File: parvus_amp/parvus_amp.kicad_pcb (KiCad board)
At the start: 2 copper layers, 86 x 60 mm, 43 parts, among them J1 input, J2 output, J3 powersupply, U1 LM3886

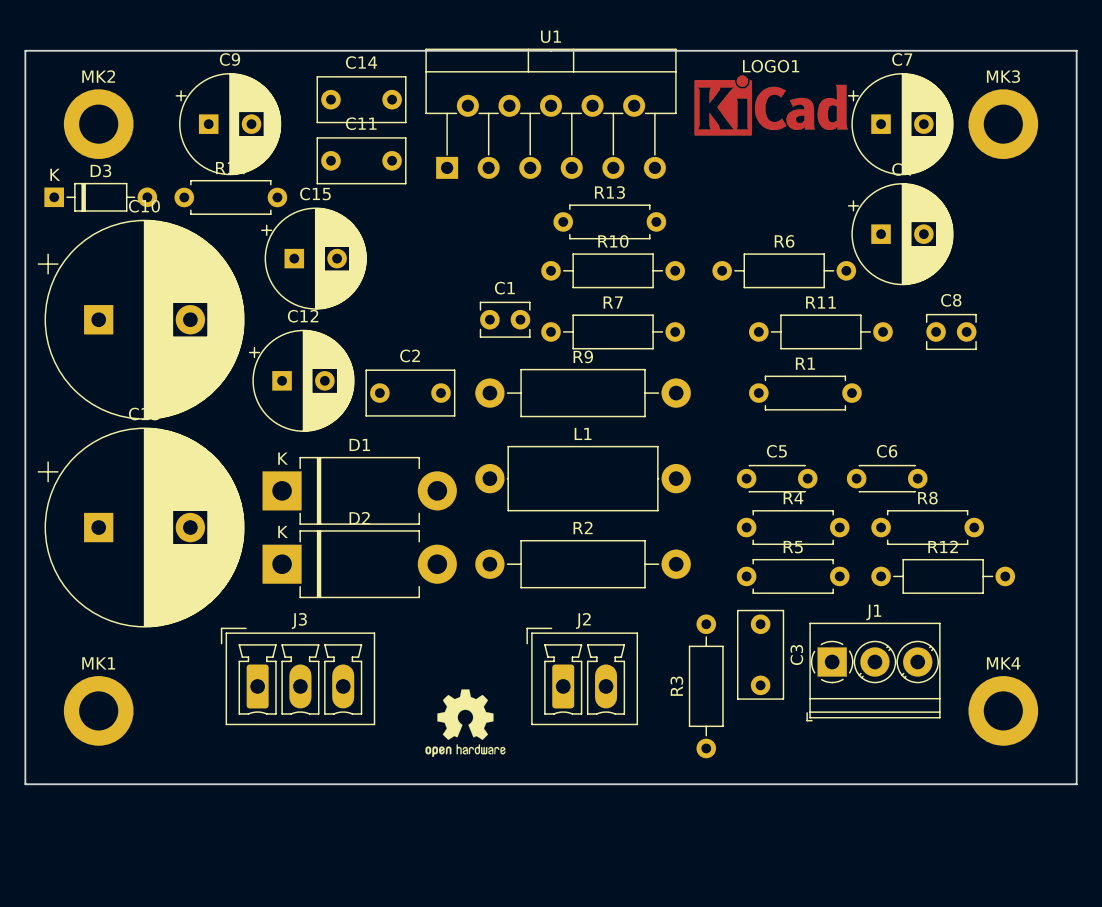
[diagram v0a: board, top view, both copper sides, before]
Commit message: Finished the amp board.
Signed-off-by: Nenad Radulovic <nenad.b.radulovic@gmail.com>
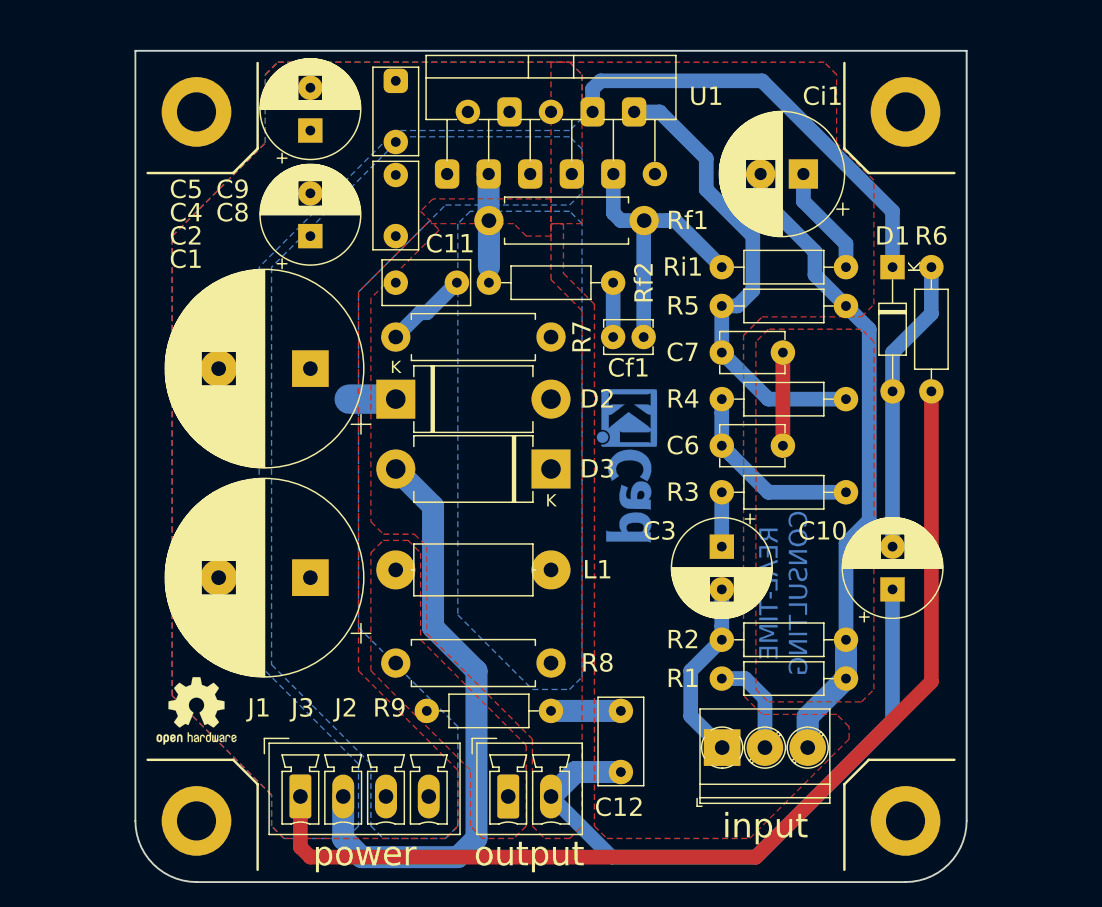
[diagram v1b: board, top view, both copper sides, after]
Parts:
- removed C13: 2m2, Capacitor_THT:CP_Radial_D16.0mm_P7.50mm
- removed C14: 100n, Capacitor_THT:C_Rect_L7.0mm_W3.5mm_P5.00mm
- removed C15: 100u, Capacitor_THT:CP_Radial_D8.0mm_P3.50mm
- removed R10: 499, Resistor_THT:R_Axial_DIN0207_L6.3mm_D2.5mm_P10.16mm_Horizontal
- removed R11: 7k5, Resistor_THT:R_Axial_DIN0207_L6.3mm_D2.5mm_P10.16mm_Horizontal
- removed R12: 10, Resistor_THT:R_Axial_DIN0207_L6.3mm_D2.5mm_P10.16mm_Horizontal
- removed R13: 1k6, Resistor_THT:R_Axial_DIN0207_L6.3mm_D2.5mm_P7.62mm_Horizontal
- removed R14: 7k5, Resistor_THT:R_Axial_DIN0207_L6.3mm_D2.5mm_P7.62mm_Horizontal
- added Cf1: 68p, Capacitor_THT:C_Disc_D3.8mm_W2.6mm_P2.50mm, F.Cu at (140.6, 76.8)
- added Ci1: 2m2, Capacitor_THT:CP_Radial_D10.0mm_P3.50mm, F.Cu at (156.1, 63.5)
- added Rf1: 1k5, Resistor_THT:R_Axial_DIN0411_L9.9mm_D3.6mm_P12.70mm_Horizontal, F.Cu at (130.4, 67.3)
- added Rf2: 430, Resistor_THT:R_Axial_DIN0207_L6.3mm_D2.5mm_P10.16mm_Horizontal, F.Cu at (140.6, 72.4)
- added Ri1: 100, Resistor_THT:R_Axial_DIN0207_L6.3mm_D2.5mm_P10.16mm_Horizontal, F.Cu at (149.5, 71.1)
- C1: value 15p -> 2m2; footprint Capacitor_THT:C_Disc_D3.8mm_W2.6mm_P2.50mm -> Capacitor_THT:CP_Radial_D16.0mm_P7.50mm
- C10: value 2m2 -> 100u; footprint Capacitor_THT:CP_Radial_D16.0mm_P7.50mm -> Capacitor_THT:CP_Radial_D8.0mm_P3.50mm
- C11: value 100n -> 220n
- C12, C9: value 100u -> 100n; footprint Capacitor_THT:CP_Radial_D8.0mm_P3.50mm -> Capacitor_THT:C_Rect_L7.0mm_W3.5mm_P5.00mm
- C2: value 220n -> 2m2; footprint Capacitor_THT:C_Rect_L7.0mm_W3.5mm_P5.00mm -> Capacitor_THT:CP_Radial_D16.0mm_P7.50mm
- C3: value 100n -> 100u; footprint Capacitor_THT:C_Rect_L7.0mm_W3.5mm_P5.00mm -> Capacitor_THT:CP_Radial_D8.0mm_P3.50mm
- C4: value 470u -> 100u
- C5: value 220p -> 100u; footprint Capacitor_THT:C_Disc_D4.3mm_W1.9mm_P5.00mm -> Capacitor_THT:CP_Radial_D8.0mm_P3.50mm
- C6: value 1n -> 2n2; footprint Capacitor_THT:C_Disc_D4.3mm_W1.9mm_P5.00mm -> Capacitor_THT:C_Disc_D5.1mm_W3.2mm_P5.00mm
- C7: value 470u -> 2n2; footprint Capacitor_THT:CP_Radial_D8.0mm_P3.50mm -> Capacitor_THT:C_Disc_D5.1mm_W3.2mm_P5.00mm
- C8: value 15p -> 100n; footprint Capacitor_THT:C_Disc_D3.8mm_W2.6mm_P2.50mm -> Capacitor_THT:C_Rect_L7.0mm_W3.5mm_P5.00mm
- D1: value 1N5404 -> BZX85C16; footprint Diode_THT:D_DO-201AD_P12.70mm_Horizontal -> Diode_THT:D_DO-35_SOD27_P10.16mm_Horizontal
- D3: value BZX85C16 -> 1N5404; footprint Diode_THT:D_DO-35_SOD27_P7.62mm_Horizontal -> Diode_THT:D_DO-201AD_P12.70mm_Horizontal
- J1: value input -> powersupply; footprint TerminalBlock_Phoenix:TerminalBlock_Phoenix_PT-1,5-3-3.5-H_1x03_P3.50mm_Horizontal -> Connector_Phoenix_MC:PhoenixContact_MCV_1,5_4-G-3.5_1x04_P3.50mm_Vertical
- J2: value output -> input; footprint Connector_Phoenix_MC:PhoenixContact_MCV_1,5_2-G-3.5_1x02_P3.50mm_Vertical -> TerminalBlock_Phoenix:TerminalBlock_Phoenix_PT-1,5-3-3.5-H_1x03_P3.50mm_Horizontal
- J3: value powersupply -> output; footprint Connector_Phoenix_MC:PhoenixContact_MCV_1,5_3-G-3.5_1x03_P3.50mm_Vertical -> Connector_Phoenix_MC:PhoenixContact_MCV_1,5_2-G-3.5_1x02_P3.50mm_Vertical
- L1: footprint Inductor_THT:L_Axial_L12.0mm_D5.0mm_P15.24mm_Horizontal_Fastron_MISC -> Inductor_THT:L_Axial_L9.5mm_D4.0mm_P12.70mm_Horizontal_Fastron_SMCC
- LOGO1: moved to B.Cu
- R1: value 1k6 -> 10; footprint Resistor_THT:R_Axial_DIN0207_L6.3mm_D2.5mm_P7.62mm_Horizontal -> Resistor_THT:R_Axial_DIN0207_L6.3mm_D2.5mm_P10.16mm_Horizontal
- R2: value 4.7 -> 100k; footprint Resistor_THT:R_Axial_DIN0411_L9.9mm_D3.6mm_P15.24mm_Horizontal -> Resistor_THT:R_Axial_DIN0207_L6.3mm_D2.5mm_P10.16mm_Horizontal
- R3: value 10 -> 100
- R4: footprint Resistor_THT:R_Axial_DIN0207_L6.3mm_D2.5mm_P7.62mm_Horizontal -> Resistor_THT:R_Axial_DIN0207_L6.3mm_D2.5mm_P10.16mm_Horizontal
- R5: value 100 -> 1k5; footprint Resistor_THT:R_Axial_DIN0207_L6.3mm_D2.5mm_P7.62mm_Horizontal -> Resistor_THT:R_Axial_DIN0207_L6.3mm_D2.5mm_P10.16mm_Horizontal
- R6: value 499 -> 7k5
- R7: value 7k5 -> 4.7; footprint Resistor_THT:R_Axial_DIN0207_L6.3mm_D2.5mm_P10.16mm_Horizontal -> Resistor_THT:R_Axial_DIN0411_L9.9mm_D3.6mm_P12.70mm_Horizontal
- R8: value 100k -> 4.7; footprint Resistor_THT:R_Axial_DIN0207_L6.3mm_D2.5mm_P7.62mm_Horizontal -> Resistor_THT:R_Axial_DIN0411_L9.9mm_D3.6mm_P12.70mm_Horizontal
- R9: value 4.7 -> 10; footprint Resistor_THT:R_Axial_DIN0411_L9.9mm_D3.6mm_P15.24mm_Horizontal -> Resistor_THT:R_Axial_DIN0207_L6.3mm_D2.5mm_P10.16mm_Horizontal
- moved C10 68.6 mm to (163.4, 97.5), turned to 90 degrees
- moved D1 53.2 mm to (163.4, 71.1), turned to 270 degrees
- moved C4 46.7 mm to (115.8, 68.6), turned to 90 degrees
- moved D3 46.3 mm to (135.5, 87.6), turned to 180 degrees
- moved C5 45.7 mm to (115.8, 59.9), turned to 90 degrees
- moved C8 44.9 mm to (122.8, 68.6), turned to 90 degrees
- moved J1 44.9 mm to (115.0, 114.4)
- moved C12 42.3 mm to (141.2, 112.4), turned to 90 degrees
- moved R8 41.2 mm to (122.8, 103.5)
- moved LOGO1 31.1 mm to (142.2, 87.4), turned to 270 degrees
- moved R9 26.5 mm to (135.5, 107.4), turned to 180 degrees
- moved C1 25.7 mm to (115.8, 96.5), turned to 180 degrees
- moved R1 24.4 mm to (159.6, 104.8), turned to 180 degrees
- moved R3 23.9 mm to (159.6, 89.5), turned to 180 degrees
- moved R5 23.6 mm to (159.6, 74.3), turned to 180 degrees
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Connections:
- C1 pad 1: Net-(C1-Pad1) -> VCC
- C1 pad 2: Net-(C1-Pad2) -> GNDPWR
- C10 pad 1: VCC -> GNDPWR
- C10 pad 2: GNDPWR -> Net-(C10-Pad2)
- C11 pad 1: VCC -> GNDPWR
- C11 pad 2: GNDPWR -> Net-(C11-Pad2)
- C12 pad 1: VCC -> GNDPWR
- C12 pad 2: GNDPWR -> Net-(C12-Pad2)
- C2 pad 1: Net-(C2-Pad1) -> GNDPWR
- C2 pad 2: Net-(C2-Pad2) -> VEE
- C4 pad 1: Net-(C4-Pad1) -> VCC
- C4 pad 2: Net-(C4-Pad2) -> GNDPWR
- C5 pad 1: Net-(C5-Pad1) -> GNDPWR
- C5 pad 2: Net-(C1-Pad1) -> VEE
- C6 pad 1: Net-(C4-Pad2) -> Net-(C6-Pad1)
- C6 pad 2: Net-(C1-Pad1) -> /sgnd
- C7 pad 2: Net-(C1-Pad1) -> /sgnd
- C8 pad 1: Net-(C2-Pad2) -> VCC
- C8 pad 2: Net-(C8-Pad2) -> GNDPWR
- C9 pad 2: Net-(C9-Pad2) -> VEE
- D1 pad 1: VCC -> Net-(D1-Pad1)
- D1 pad 2: Net-(C2-Pad2) -> Net-(C10-Pad2)
- D2 pad 1: Net-(C2-Pad2) -> VCC
- D2 pad 2: VEE -> /out
- D3 pad 1: Net-(D3-Pad1) -> /out
- D3 pad 2: Net-(C9-Pad2) -> VEE
- J1 pad 2: GNDPWR -> VEE
- J1 pad 3: Net-(C1-Pad1) -> GNDPWR
- J2 pad 1: GNDPWR -> Net-(C3-Pad2)
- J2 pad 2: Net-(C3-Pad2) -> GNDPWR
- J3 pad 1: VCC -> Net-(J3-Pad1)
- L1 pad 1: Net-(C2-Pad2) -> /out
- L1 pad 2: Net-(C3-Pad2) -> Net-(J3-Pad1)
- R1 pad 1: Net-(R1-Pad1) -> /sgnd
- R1 pad 2: Net-(C1-Pad2) -> GNDPWR
- R2 pad 1: GNDPWR -> Net-(C3-Pad2)
- R2 pad 2: Net-(C2-Pad1) -> /sgnd
- R3 pad 1: GNDPWR -> Net-(C6-Pad1)
- R4 pad 1: Net-(C5-Pad1) -> Net-(C7-Pad1)
- R4 pad 2: Net-(J1-Pad1) -> Net-(C6-Pad1)
- R5 pad 1: Net-(C4-Pad2) -> /sgnd
- R5 pad 2: Net-(C5-Pad1) -> Net-(C7-Pad1)
- R6 pad 1: Net-(R1-Pad1) -> Net-(C10-Pad2)
- R6 pad 2: Net-(C4-Pad1) -> Net-(J1-Pad1)
- R7 pad 1: Net-(C1-Pad1) -> Net-(C11-Pad2)
- R7 pad 2: Net-(R1-Pad1) -> /out
- R8 pad 1: Net-(J1-Pad1) -> Net-(J3-Pad1)
- R8 pad 2: Net-(C1-Pad1) -> /out
- R9 pad 1: Net-(C3-Pad2) -> Net-(C12-Pad2)
- R9 pad 2: Net-(C2-Pad2) -> Net-(J3-Pad1)
- U1 pad 10: Net-(R1-Pad1) -> Net-(C7-Pad1)
- U1 pad 3: Net-(C2-Pad2) -> /out
- U1 pad 8: Net-(D3-Pad1) -> Net-(D1-Pad1)
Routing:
- net Net-(J1-Pad1): track 0.00 -> 85.8 mm
- net /sgnd: track 0.00 -> 60.3 mm
- net GNDPWR: track 0.00 -> 60.1 mm
- net VEE: track 0.00 -> 48.6 mm
- net Net-(C7-Pad1): track 0.00 -> 38.5 mm
- net Net-(D1-Pad1): track 0.00 -> 35.7 mm
- net Net-(C10-Pad2): track 0.00 -> 24.2 mm
- net Net-(Cf1-Pad2): track 0.00 -> 23.4 mm
- net Net-(C6-Pad1): track 0.00 -> 15.5 mm
- net Net-(C3-Pad2): track 0.00 -> 15.1 mm
- net Net-(Ci1-Pad1): track 0.00 -> 9.06 mm
- net /out: track 0.00 -> 7.66 mm
- net Net-(C11-Pad2): track 0.00 -> 6.84 mm
- net Net-(C12-Pad2): track 0.00 -> 5.72 mm
- net Net-(C3-Pad1): track 0.00 -> 4.45 mm
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- added copper zone on B.Cu, net /out
- added copper zone on F.Cu, net /sgnd
- added copper zone on F.Cu, net GNDPWR
- added copper zone on F.Cu, net Net-(J3-Pad1)
- added copper zone on B.Cu, net VCC
- added copper zone on B.Cu, net VEE
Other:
- board size 86 x 60 mm -> 68 x 68 mm
- net class Default: clearance 0.2 -> 0.254; trace_width 0.25 -> 1
- rule trace_clearance: 0.2 -> 0.254
- board text added: "+/PG/-/mute"
- board text added: "190523"
- board text added: "PG/out"
- board text added: "REAL-TIME CONSULTING"
- board text added: "SG/PG/in"
- board text added: "input"
- board text added: "output"
- board text added: "parvus v1.0"
- board text added: "power"
